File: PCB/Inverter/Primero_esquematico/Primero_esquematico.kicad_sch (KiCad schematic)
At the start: 0 parts

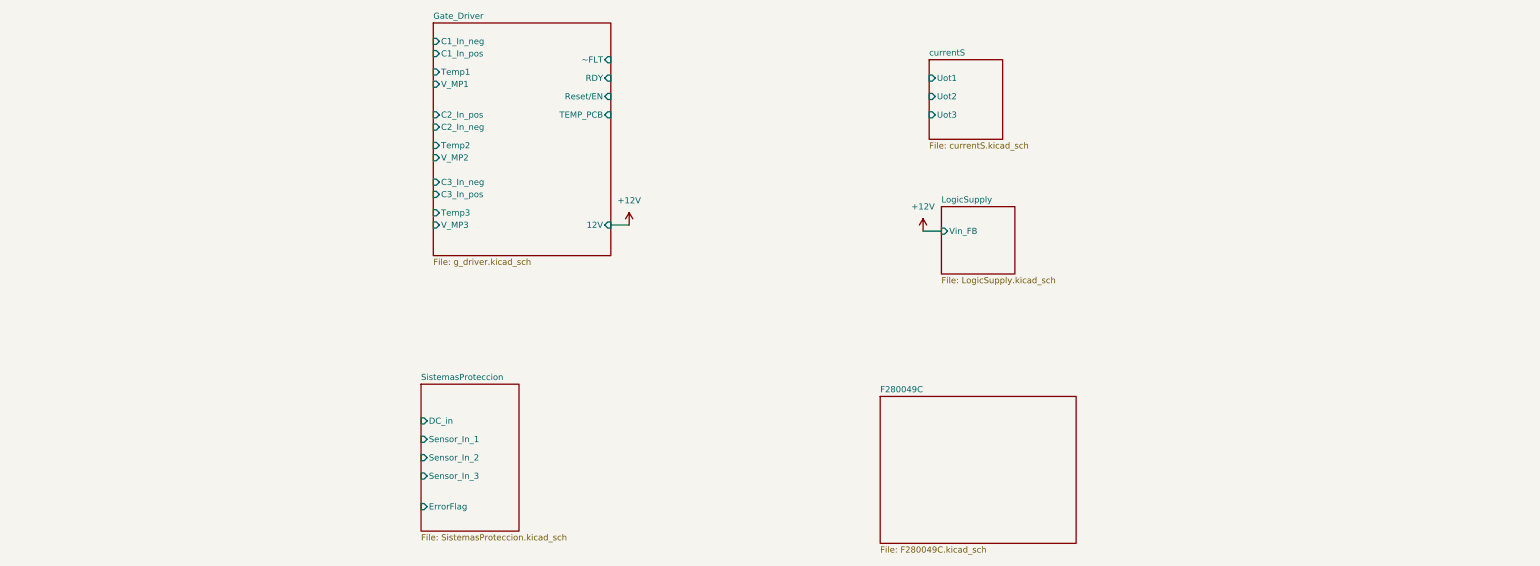
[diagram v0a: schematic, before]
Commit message: Esquematico practicamente terminado
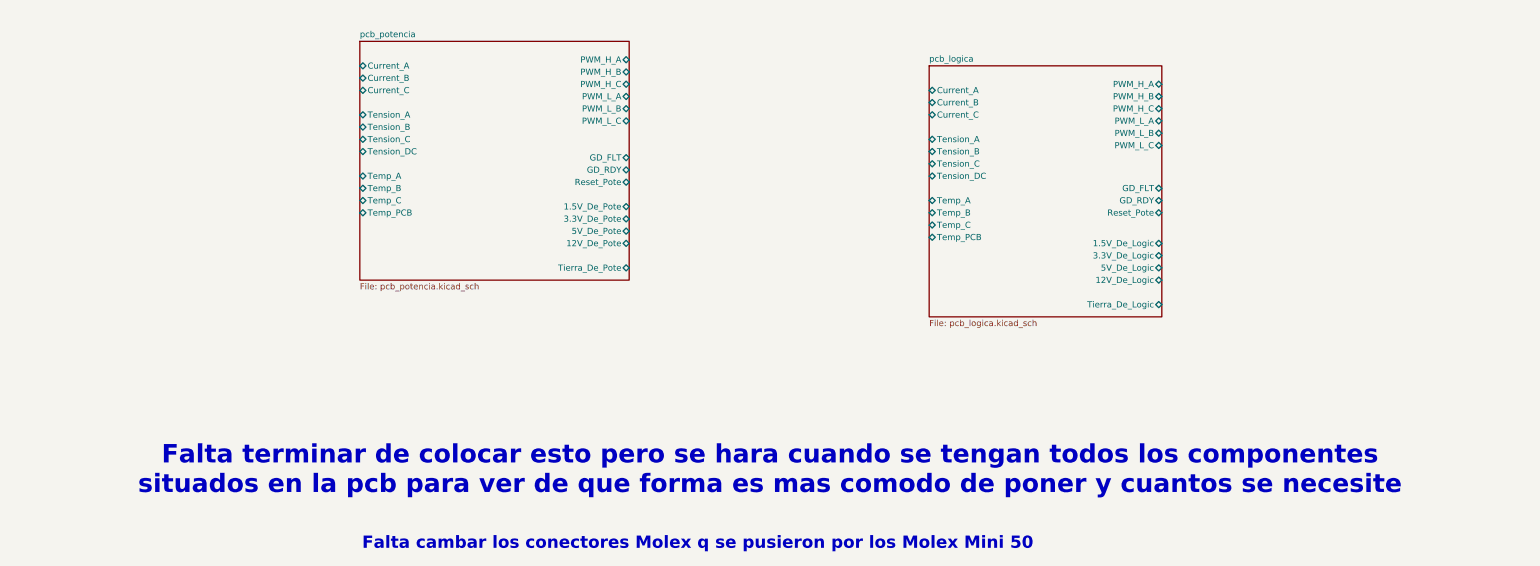
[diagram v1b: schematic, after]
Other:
- removed sheet F280049C
- removed sheet Gate_Driver
- removed sheet LogicSupply
- removed sheet SistemasProteccion
- removed sheet currentS
- added sheet pcb_logica (pcb_logica.kicad_sch)
- added sheet pcb_potencia (pcb_potencia.kicad_sch)
- note added: "Falta cambar los conectores Molex q se pusieron por los Molex Mini 50"
- note added: "Falta terminar de colocar esto pero se hara cuando se tengan todos los componentes situados en la pcb para ver de que forma es mas comodo de poner y cuantos se necesite"
